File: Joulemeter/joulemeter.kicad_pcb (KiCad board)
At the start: 2 copper layers, 129.5 x 83.5 mm, 50 parts, among them J1 XT60-M, J2 XT60-M, J3 22035035, J4 22035035, U2 MCP6286T-E/OT, U5 PADS131M04QPWRQ1

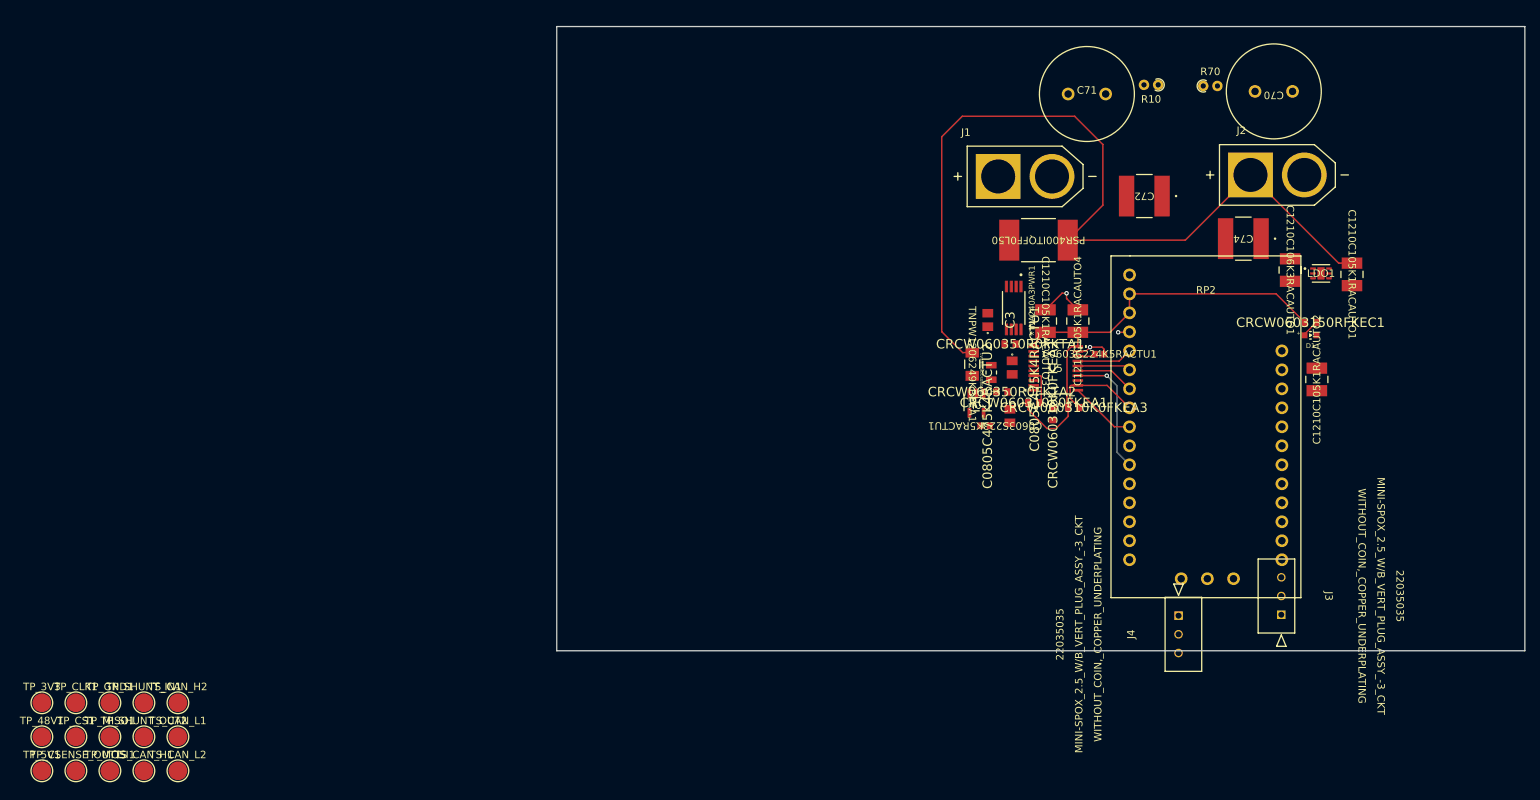
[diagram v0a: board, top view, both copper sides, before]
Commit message: pcb changes 2
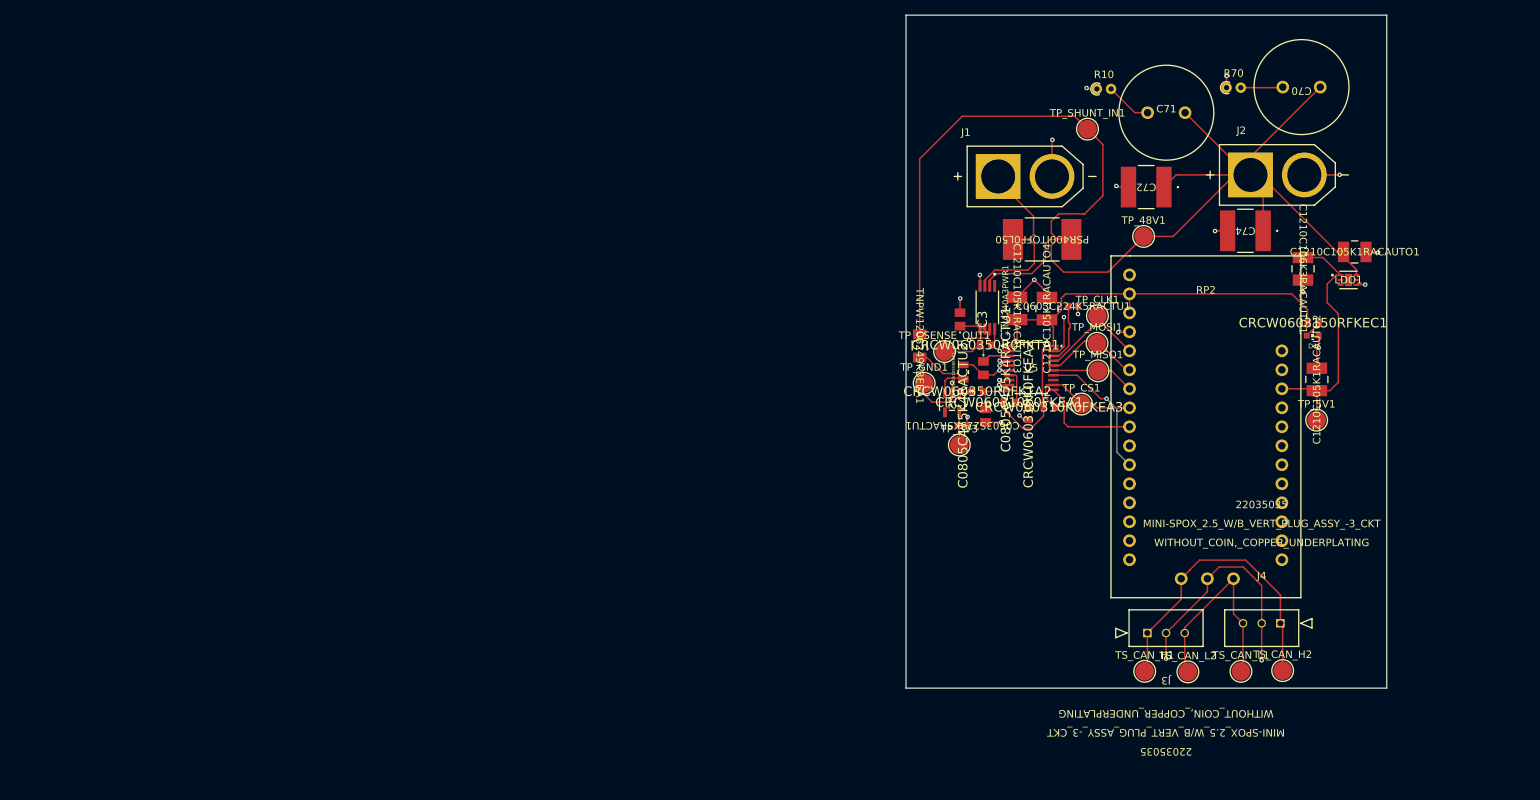
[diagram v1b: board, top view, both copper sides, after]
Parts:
- removed TP_SHUNT_OUT2: ~, TestPoint:TestPoint_Pad_D2.5mm
- moved TP_5V1 176.9 mm to (184.2, 108.2)
- moved TP_48V1 161.9 mm to (161.0, 83.6)
- moved TS_CAN_H2 147.8 mm to (179.6, 141.7)
- moved TP_SHUNT_IN1 147.7 mm to (153.5, 69.2)
- moved TP_CLK1 146.1 mm to (154.8, 94.2)
- moved TP_MOSI1 143.9 mm to (154.8, 97.9)
- moved TS_CAN_L1 142.5 mm to (174.0, 141.8)
- moved TP_CS1 141.7 mm to (152.7, 106.0)
- moved TP_MISO1 140.9 mm to (154.9, 101.5)
- moved TS_CAN_L2 135.7 mm to (166.9, 141.8)
- moved TS_CAN_H1 134.5 mm to (161.2, 141.8)
- moved TP_CSENSE_OUT1 129.0 mm to (134.4, 99.0)
- moved TP_3V3 127.5 mm to (136.3, 111.5)
- moved TP_GND1 117.0 mm to (131.7, 103.2)
- moved J3 18.1 mm to (161.5, 136.6), turned to 180 degrees
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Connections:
- C70 pad 3: (no net) -> Net-(C70-Pad1)
- C70 pad 4: (no net) -> +48V
- C71 pad 3: (no net) -> +48V
- C71 pad 4: (no net) -> Net-(C71-Pad1)
- C74 pad 1: Net-(J2-POS) -> +48V
- RP2 pad 1: /CAN_H -> (no net)
- RP2 pad 2: GND -> (no net)
- RP2 pad 29: (no net) -> /CAN_L
- RP2 pad 30: (no net) -> GND
- RP2 pad 31: (no net) -> /CAN_H
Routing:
- net GND: track 13.7 -> 105.8 mm, vias 3 -> 29
- net +48V: track 116.8 -> 199.1 mm
- net /CAN_H: track 0.00 -> 40.9 mm
- net +5V: track 0.06 -> 34.1 mm
- net /SHUNT_LOAD: track 4.01 -> 33.6 mm
- net /CAN_L: track 0.00 -> 28.4 mm
- net +3V3: track 62.9 -> 80.9 mm
- net Net-(U2-VIN+): track 0.00 -> 11.3 mm
- net /CSENSE_OUT: track 0.00 -> 11.2 mm
- net /GPIO_CLKIN: track 7.48 -> 15.3 mm
- net /MOSI: track 7.13 -> 13.6 mm
- net Net-(C71-Pad1): track 0.00 -> 6.20 mm
- net /Vdivider: track 0.00 -> 6.05 mm
- net Net-(U5-CAP): track 2.38 -> 8.08 mm
- net Net-(C70-Pad1): track 0.00 -> 5.65 mm
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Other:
- board size 129.5 x 83.5 mm -> 64.3 x 90 mm

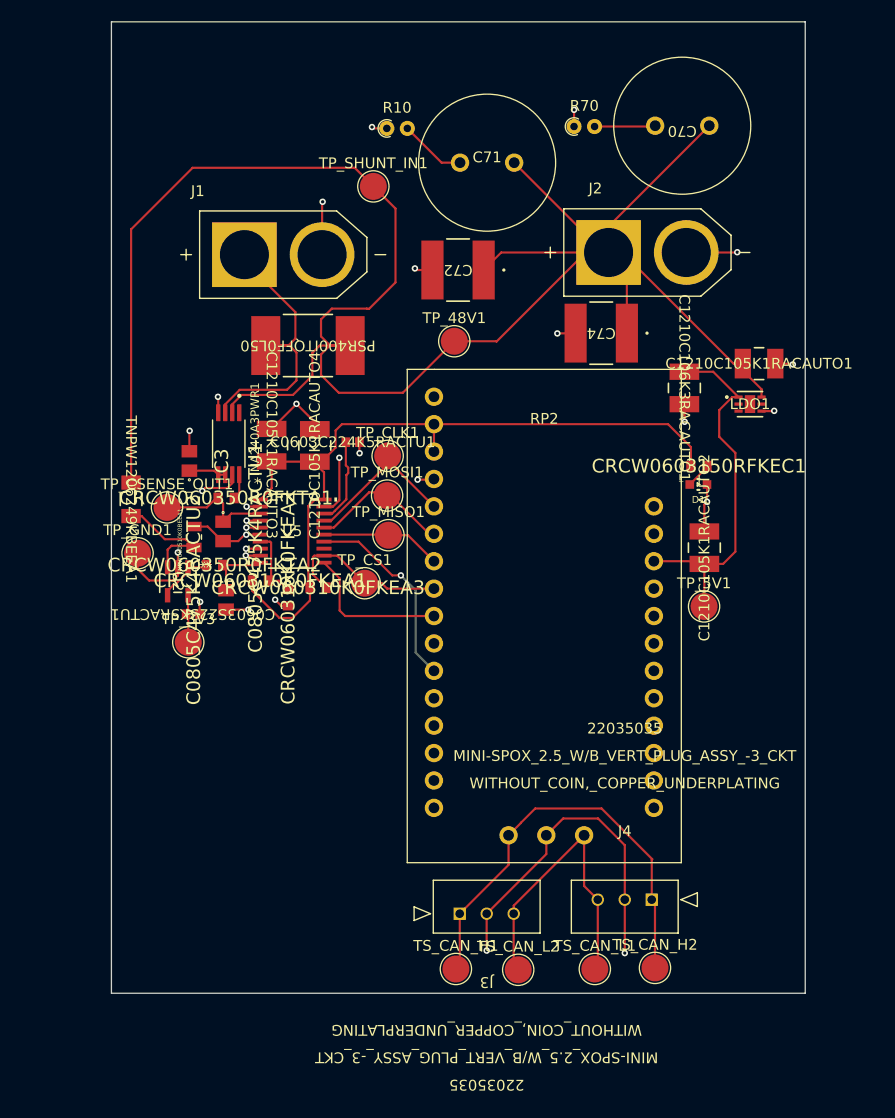
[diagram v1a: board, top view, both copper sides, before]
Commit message: pcb 4
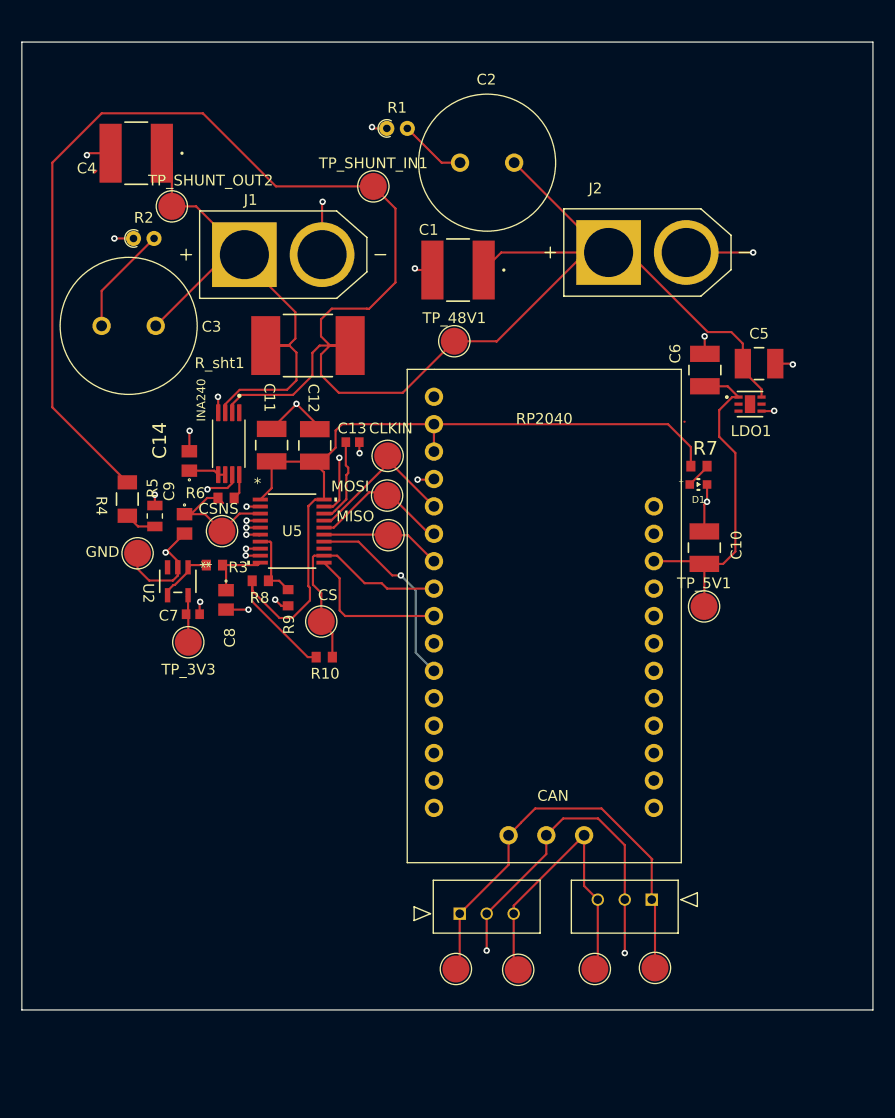
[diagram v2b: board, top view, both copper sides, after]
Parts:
- added TP_SHUNT_OUT2: ~, TestPoint:TestPoint_Pad_D2.5mm, F.Cu at (134.8, 71.1)
- C1: renamed from C72; value C2220C475M1R2C7186 -> 4.7 µF
- C10: renamed from C1210C105K1RACAUTO2; value 1μF -> 1 µF
- C4: renamed from C74; value C2220C475M1R2C7186 -> 4.7 µF
- moved C3 54.6 mm to (130.8, 82.2)
- moved C4 46.2 mm to (131.5, 66.2)
- moved R2 42.1 mm to (131.3, 74.0)
- moved R10 6.46 mm to (148.9, 112.8)
- moved CSNS 5.55 mm to (139.5, 101.2)
- moved CS 5.37 mm to (148.7, 109.5)
- moved R5 4.12 mm to (133.2, 99.8)
- moved C9 3.64 mm to (136.0, 100.5)
- moved C6 2.52 mm to (184.2, 86.2), turned to 90 degrees
- moved R4 0.35 mm to (130.7, 98.2)
- renumbered C1210C105K1RACAUTO3 to C11, C1210C105K1RACAUTO4 to C12, C0603C224K5RACTU1 to C13, C3 to C14, C71 to C2, C70 to C3, C1210C105K1RACAUTO1 to C5, C1210C106K3RACAUTO1 to C6, C0603S223K5RACTU1 to C7, C0805C475K4RACTU2 to C8, C0805C475K4RACTU1 to C9, J4 to CAN, TP_CLK1 to CLKIN, TP_CS1 to CS, TP_CSENSE_OUT1 to CSNS, TP_GND1 to GND, INA240A3PWR1 to INA240, TP_MISO1 to MISO, TP_MOSI1 to MOSI, R10 to R1, CRCW060310K0FKEA3 to R10, R70 to R2, CRCW060350R0FKTA2 to R3, TNPW1206249KBEEA1 to R4, TNPW080510K0BEEA1 to R5, CRCW060350R0FKTA1 to R6, CRCW0603150RFKEC1 to R7, CRCW060310K0FKEA1 to R8, CRCW060310K0FKEA2 to R9, RP2 to RP2040, PSR400ITQFF0L50 to R_sht1
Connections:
- C2 pad 3: +48V -> (no net)
- C2 pad 4: Net-(C71-Pad1) -> (no net)
- C3 pad 4: +48V -> /SHUNT_LOAD
- C4 pad 1: +48V -> /SHUNT_LOAD
- R1 pad 2: Net-(C71-Pad1) -> Net-(C2-Pad1)
- RP2040 pad 1: (no net) -> /CAN_H
- RP2040 pad 2: (no net) -> GND
- RP2040 pad 29: /CAN_L -> (no net)
- RP2040 pad 30: GND -> (no net)
- RP2040 pad 31: /CAN_H -> (no net)
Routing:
- net /SHUNT_LOAD: track 33.6 -> 58.4 mm
- net +3V3: track 80.9 -> 90.9 mm
- net Net-(U2-VIN+): track 11.3 -> 2.96 mm
- net /CS: track 15.9 -> 22.6 mm
- net Net-(C71-Pad1): track 6.20 -> 0.00 mm
- net Net-(C2-Pad1): track 0.00 -> 6.20 mm
- net Net-(C3-Pad1): track 5.65 -> 10.1 mm
- net +5V: track 34.1 -> 31.7 mm
- net /CSENSE_OUT: track 11.2 -> 13.0 mm
- net GND: track 105.8 -> 106.1 mm, vias 29 -> 30
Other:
- board size 64.3 x 90 mm -> 78.9 x 89.7 mm
